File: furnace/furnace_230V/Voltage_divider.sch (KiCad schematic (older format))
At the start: 14 parts

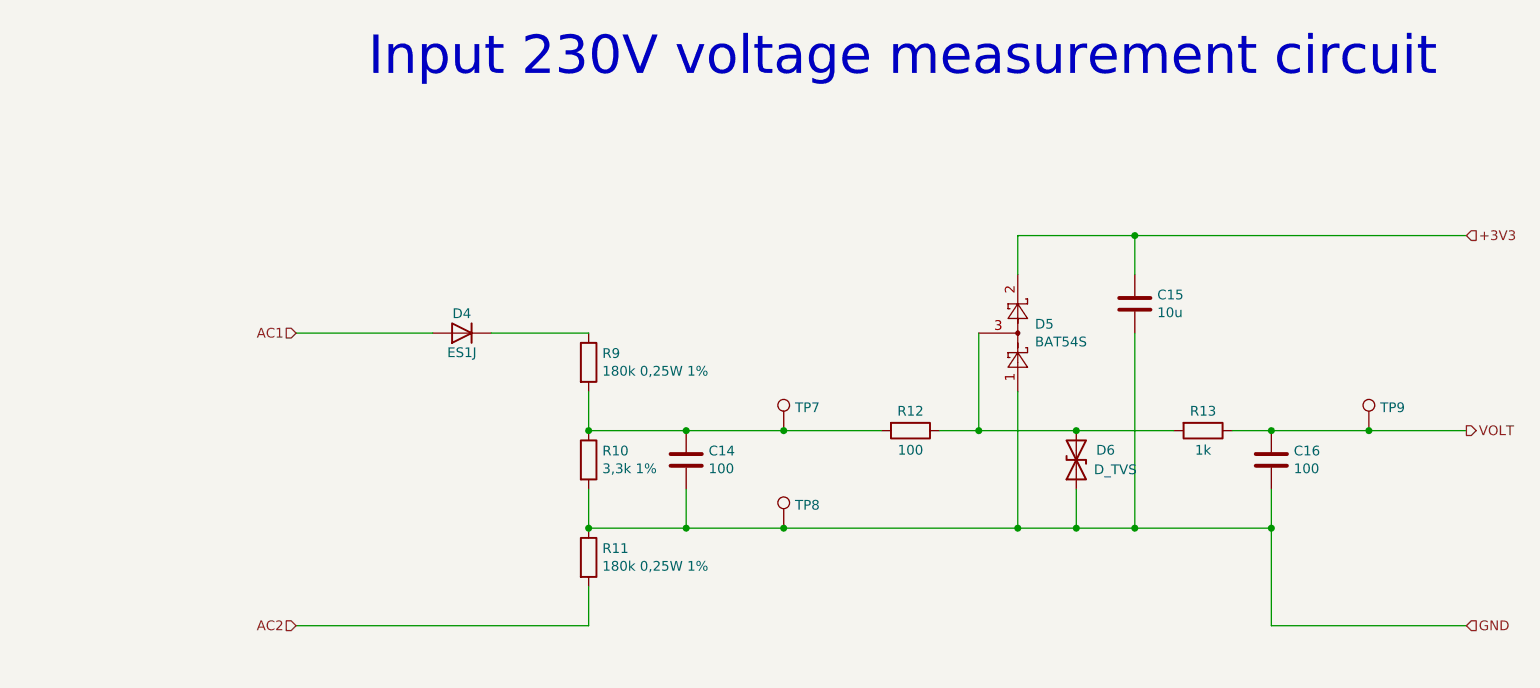
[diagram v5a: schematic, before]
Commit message: Add files via upload
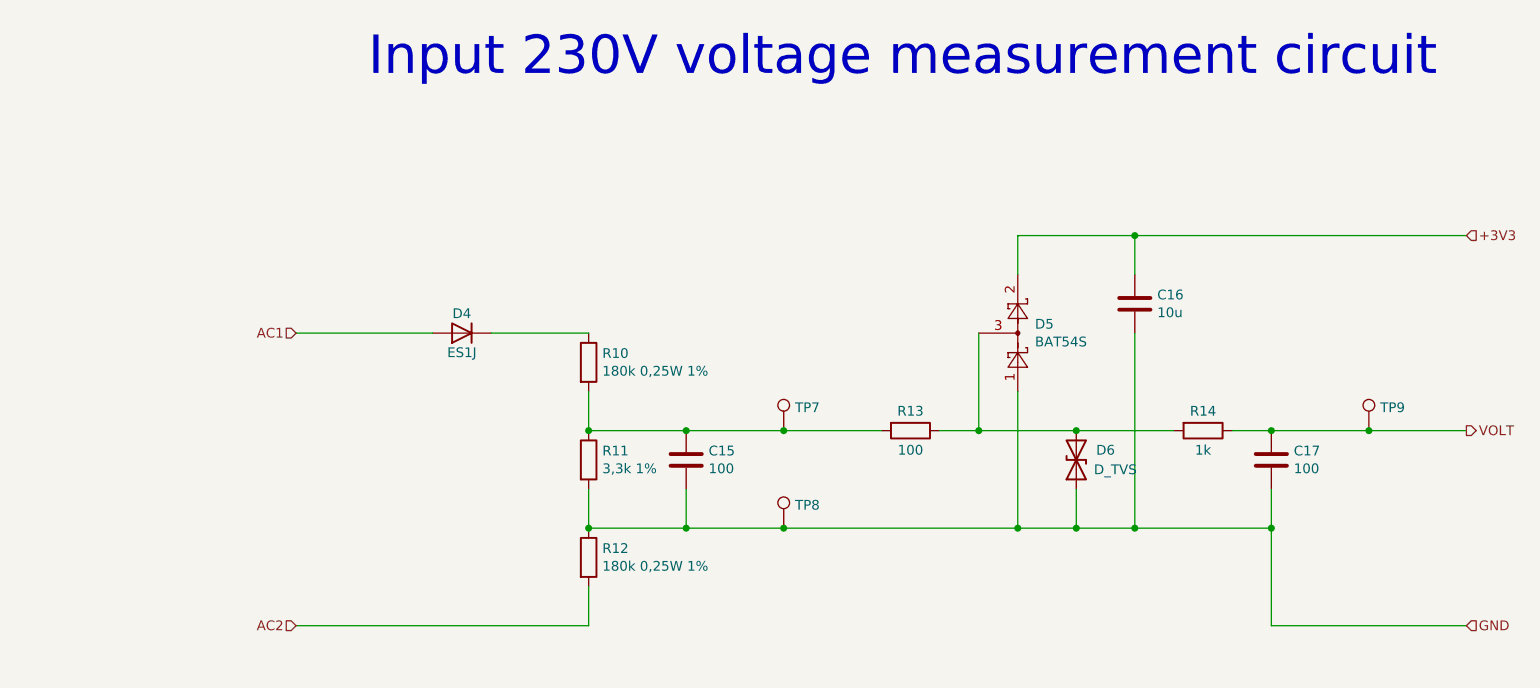
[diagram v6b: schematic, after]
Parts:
- C15: renamed from C14; footprint Capacitor_SMD:C_0603_1608Metric_Pad1.05x0.95mm_HandSolder -> Capacitor_SMD:C_0603_1608Metric_Pad1.08x0.95mm_HandSolder
- C16: renamed from C15; footprint Capacitor_SMD:C_0603_1608Metric_Pad1.05x0.95mm_HandSolder -> Capacitor_SMD:C_0603_1608Metric_Pad1.08x0.95mm_HandSolder
- C17: renamed from C16; footprint Capacitor_SMD:C_0603_1608Metric_Pad1.05x0.95mm_HandSolder -> Capacitor_SMD:C_0603_1608Metric_Pad1.08x0.95mm_HandSolder
- D4: footprint Diode_SMD:D_SMA_Handsoldering -> Diode_SMD:D_SMA-SMB_Universal_Handsoldering
- D6: footprint Diode_SMD:D_SMB_Handsoldering -> Diode_SMD:D_SMA-SMB_Universal_Handsoldering
- R11: renamed from R10; footprint Resistor_SMD:R_0603_1608Metric_Pad1.05x0.95mm_HandSolder -> Resistor_SMD:R_0603_1608Metric_Pad0.98x0.95mm_HandSolder
- TP7, TP8, TP9: footprint furnace_230V:TP -> MountingHole:MountingHole_2.2mm_M2_DIN965_Pad_TopBottom
- renumbered R9 to R10, R11 to R12, R12 to R13, R13 to R14
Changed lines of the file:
@@
 P 4500 3650
 AR Path="/60AAE0B8/60AC3251" Ref="R?"  Part="1"
-AR Path="/60AAE4BD/60AC3251" Ref="R9"  Part="1"
-F 0 "R9" H 4570 3696 50  0000 L CNN
+AR Path="/60AAE4BD/60AC3251" Ref="R10"  Part="1"
+F 0 "R10" H 4570 3696 50  0000 L CNN
 F 1 "180k 0,25W 1%" H 4570 3605 50  0000 L CNN
 F 2 "Resistor_THT:R_Axial_DIN0207_L6.3mm_D2.5mm_P10.16mm_Horizontal" V 4430 3650 50  0001 C CNN
@@
 AR Path="/60AAE0B8/60AC39AB" Ref="R?"  Part="1"
 AR Path="/60AAEC6C/60AC39AB" Ref="R?"  Part="1"
-AR Path="/60AAE4BD/60AC39AB" Ref="R12"  Part="1"
-F 0 "R12" V 6050 4000 50  0000 C CNN
+AR Path="/60AAE4BD/60AC39AB" Ref="R13"  Part="1"
+F 0 "R13" V 6050 4000 50  0000 C CNN
 F 1 "100" V 6250 4000 50  0000 C CNN
 F 2 "Resistor_SMD:R_0603_1608Metric_Pad1.05x0.95mm_HandSolder" V 6080 4000 50  0001 C CNN
@@
 F 0 "D6" V 7050 4000 50  0000 C CNN
 F 1 "D_TVS" V 6950 3950 50  0000 C CNN
-F 2 "Diode_SMD:D_SMB_Handsoldering" H 7000 4150 50  0001 C CNN
+F 2 "Diode_SMD:D_SMA-SMB_Universal_Handsoldering" H 7000 4150 50  0001 C CNN
 F 3 "~" H 7000 4150 50  0001 C CNN
 	1    7000 4150
@@
 AR Path="/60AAE0B8/60AC5A68" Ref="R?"  Part="1"
 AR Path="/60AAEC6C/60AC5A68" Ref="R?"  Part="1"
-AR Path="/60AAE4BD/60AC5A68" Ref="R13"  Part="1"
-F 0 "R13" V 7550 4000 50  0000 C CNN
+AR Path="/60AAE4BD/60AC5A68" Ref="R14"  Part="1"
+F 0 "R14" V 7550 4000 50  0000 C CNN
 F 1 "1k" V 7750 4000 50  0000 C CNN
 F 2 "Resistor_SMD:R_0603_1608Metric_Pad1.05x0.95mm_HandSolder" V 7580 4000 50  0001 C CNN
@@
 AR Path="/609CA6A8/60AE5653/60AC6425" Ref="C?"  Part="1"
 AR Path="/60AAC605/60AC6425" Ref="C?"  Part="1"
-AR Path="/60AAE4BD/60AC6425" Ref="C16"  Part="1"
-F 0 "C16" H 8115 4196 50  0000 L CNN
+AR Path="/60AAE4BD/60AC6425" Ref="C17"  Part="1"
+F 0 "C17" H 8115 4196 50  0000 L CNN
 F 1 "100" H 8115 4105 50  0000 L CNN
-F 2 "Capacitor_SMD:C_0603_1608Metric_Pad1.05x0.95mm_HandSolder" H 8038 4000 50  0001 C CNN
+F 2 "Capacitor_SMD:C_0603_1608Metric_Pad1.08x0.95mm_HandSolder" H 8038 4000 50  0001 C CNN
 F 3 "~" H 8000 4150 50  0001 C CNN
 	1    8000 4150
@@
 F 0 "TP7" H 5558 4118 50  0000 L CNN
 F 1 "TestPoint" H 5558 4027 50  0001 L CNN
-F 2 "furnace_230V:TP" H 5700 4000 50  0001 C CNN
+F 2 "MountingHole:MountingHole_2.2mm_M2_DIN965_Pad_TopBottom" H 5700 4000 50  0001 C CNN
 F 3 "~" H 5700 4000 50  0001 C CNN
 	1    5500 4000
@@
 F 0 "TP8" H 5558 4618 50  0000 L CNN
 F 1 "TestPoint" H 5558 4527 50  0001 L CNN
-F 2 "furnace_230V:TP" H 5700 4500 50  0001 C CNN
+F 2 "MountingHole:MountingHole_2.2mm_M2_DIN965_Pad_TopBottom" H 5700 4500 50  0001 C CNN
 F 3 "~" H 5700 4500 50  0001 C CNN
 	1    5500 4500
@@
 F 0 "TP9" H 8558 4118 50  0000 L CNN
 F 1 "TestPoint" H 8558 4027 50  0001 L CNN
-F 2 "furnace_230V:TP" H 8700 4000 50  0001 C CNN
+F 2 "MountingHole:MountingHole_2.2mm_M2_DIN965_Pad_TopBottom" H 8700 4000 50  0001 C CNN
 F 3 "~" H 8700 4000 50  0001 C CNN
 	1    8500 4000
@@
 AR Path="/609CA6A8/60AE5653/60B35196" Ref="C?"  Part="1"
 AR Path="/60AAC605/60B35196" Ref="C?"  Part="1"
-AR Path="/60AAE4BD/60B35196" Ref="C14"  Part="1"
-F 0 "C14" H 5115 4196 50  0000 L CNN
+AR Path="/60AAE4BD/60B35196" Ref="C15"  Part="1"
+F 0 "C15" H 5115 4196 50  0000 L CNN
 F 1 "100" H 5115 4105 50  0000 L CNN
-F 2 "Capacitor_SMD:C_0603_1608Metric_Pad1.05x0.95mm_HandSolder" H 5038 4000 50  0001 C CNN
+F 2 "Capacitor_SMD:C_0603_1608Metric_Pad1.08x0.95mm_HandSolder" H 5038 4000 50  0001 C CNN
 F 3 "~" H 5000 4150 50  0001 C CNN
 	1    5000 4150
@@
 AR Path="/60AAC605/60B367EA" Ref="R?"  Part="1"
 AR Path="/60AAE178/60B367EA" Ref="R?"  Part="1"
-AR Path="/60AAE4BD/60B367EA" Ref="R10"  Part="1"
-F 0 "R10" H 4570 4196 50  0000 L CNN
+AR Path="/60AAE4BD/60B367EA" Ref="R11"  Part="1"
+F 0 "R11" H 4570 4196 50  0000 L CNN
 F 1 "3,3k 1%" H 4570 4105 50  0000 L CNN
-F 2 "Resistor_SMD:R_0603_1608Metric_Pad1.05x0.95mm_HandSolder" V 4430 4150 50  0001 C CNN
+F 2 "Resistor_SMD:R_0603_1608Metric_Pad0.98x0.95mm_HandSolder" V 4430 4150 50  0001 C CNN
 F 3 "~" H 4500 4150 50  0001 C CNN
 	1    4500 4150
@@
 P 4500 4650
 AR Path="/60AAE0B8/60B376FC" Ref="R?"  Part="1"
-AR Path="/60AAE4BD/60B376FC" Ref="R11"  Part="1"
-F 0 "R11" H 4570 4696 50  0000 L CNN
+AR Path="/60AAE4BD/60B376FC" Ref="R12"  Part="1"
+F 0 "R12" H 4570 4696 50  0000 L CNN
 F 1 "180k 0,25W 1%" H 4570 4605 50  0000 L CNN
 F 2 "Resistor_THT:R_Axial_DIN0207_L6.3mm_D2.5mm_P10.16mm_Horizontal" V 4430 4650 50  0001 C CNN
@@
 AR Path="/609CA6A8/60AE5653/60B3D4CA" Ref="C?"  Part="1"
 AR Path="/60AAC605/60B3D4CA" Ref="C?"  Part="1"
-AR Path="/60AAE4BD/60B3D4CA" Ref="C15"  Part="1"
-F 0 "C15" H 7415 3396 50  0000 L CNN
+AR Path="/60AAE4BD/60B3D4CA" Ref="C16"  Part="1"
+F 0 "C16" H 7415 3396 50  0000 L CNN
 F 1 "10u" H 7415 3305 50  0000 L CNN
-F 2 "Capacitor_SMD:C_0603_1608Metric_Pad1.05x0.95mm_HandSolder" H 7338 3200 50  0001 C CNN
+F 2 "Capacitor_SMD:C_0603_1608Metric_Pad1.08x0.95mm_HandSolder" H 7338 3200 50  0001 C CNN
 F 3 "~" H 7300 3350 50  0001 C CNN
 	1    7300 3350
@@
 F 0 "D4" H 3850 3400 50  0000 C CNN
 F 1 "ES1J" H 3850 3600 50  0000 C CNN
-F 2 "Diode_SMD:D_SMA_Handsoldering" H 3850 3500 50  0001 C CNN
+F 2 "Diode_SMD:D_SMA-SMB_Universal_Handsoldering" H 3850 3500 50  0001 C CNN
 F 3 "~" H 3850 3500 50  0001 C CNN
 	1    3850 3500
